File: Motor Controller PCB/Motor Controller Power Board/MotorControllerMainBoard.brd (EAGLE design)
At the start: 70 x 100 mm, 47 parts

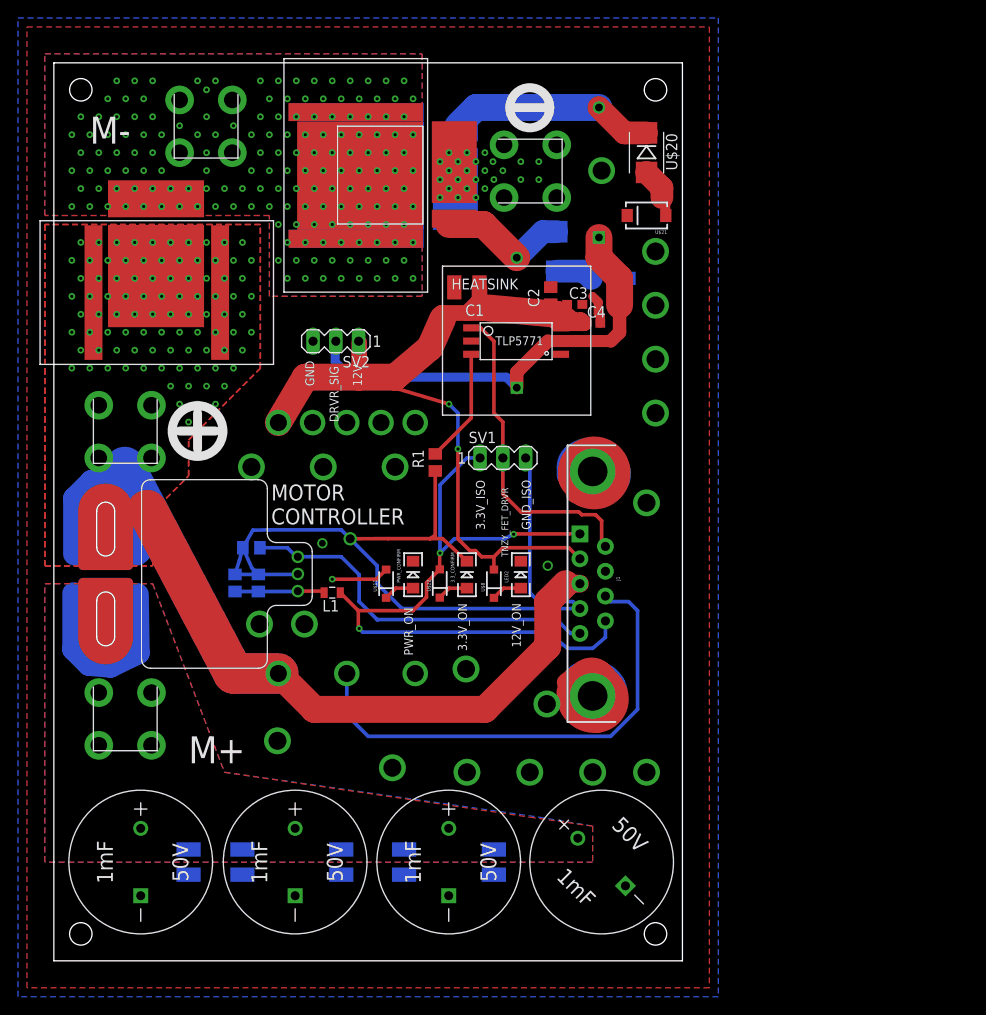
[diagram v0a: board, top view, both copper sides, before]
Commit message: Finishing Touches
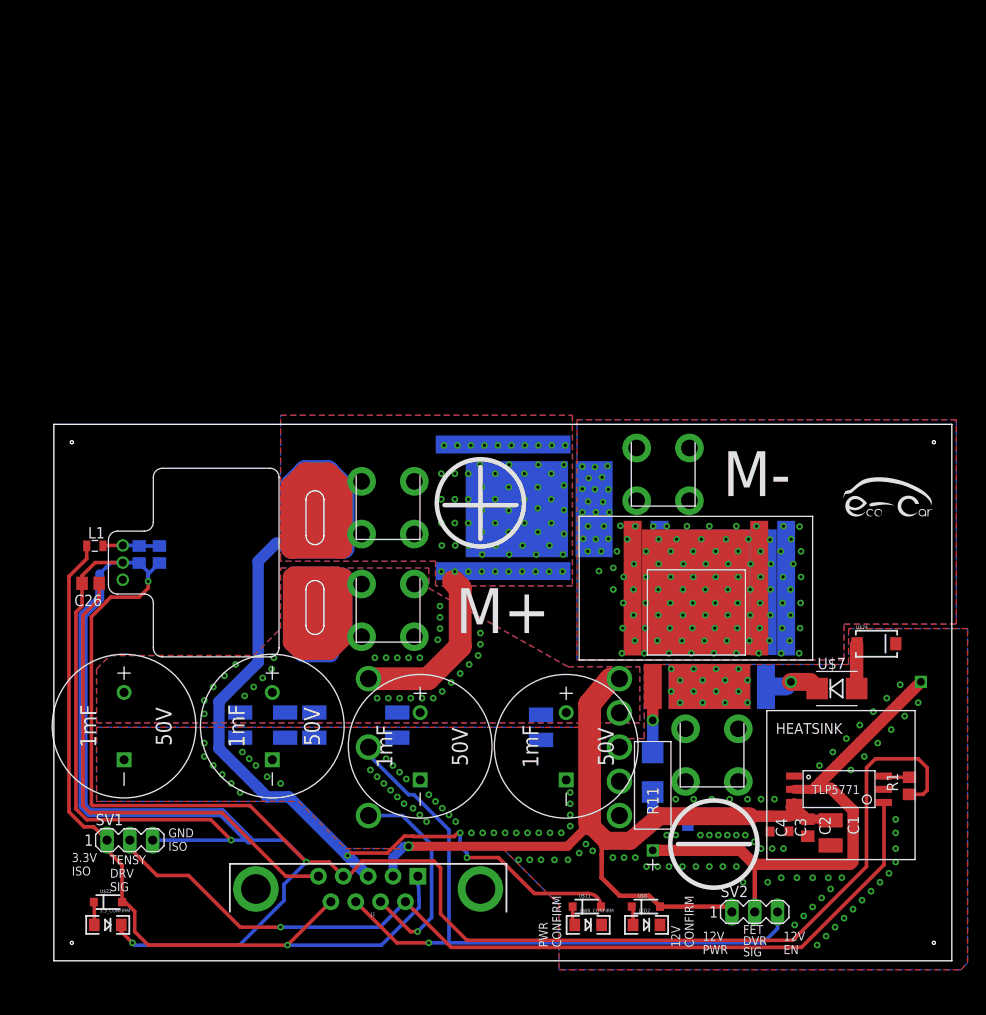
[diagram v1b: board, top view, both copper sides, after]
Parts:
- added U$26: (no value), Shell2015:LOGO
- moved SV2 78.8 mm to (78.0, 5.44), turned to 0 degrees
- moved C1 73.0 mm to (86.5, 14.2), turned to 270 degrees
- moved U$20 69.0 mm to (66.7, 21.0), flipped to the bottom
- moved R11 68.5 mm to (66.7, 26.8), flipped to the top
- moved U$21 67.9 mm to (68.5, 15.2), flipped to the bottom
- moved U$15 66.6 mm to (70.3, 20.0), turned to 0 degrees
- moved C2 65.8 mm to (84.0, 14.8), turned to 270 degrees
- moved U$12 64.0 mm to (64.9, 51.2)
- moved R1 63.9 mm to (95.3, 19.5)
- moved C3 62.6 mm to (81.9, 15.3), turned to 270 degrees
- moved U$2 61.7 mm to (74.5, 39.8), flipped to the bottom, turned to 0 degrees
- moved U$4 61.5 mm to (74.5, 41.5), flipped to the bottom, turned to 0 degrees
- moved U$25 61.3 mm to (79.4, 11.3)
- moved U$1 59.8 mm to (71.5, 39.8), flipped to the top, turned to 0 degrees
- moved U$3 59.5 mm to (71.5, 41.5), flipped to the top, turned to 0 degrees
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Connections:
- net ENABLE_12V: now also SV2.3
- net GND: no longer SV2.3
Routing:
- net GND_ISOLATED: track 100.4 -> 304.8 mm, vias 1 -> 4
- net TEENSY_FET_DRIVER_SIGNAL: track 35.8 -> 102.5 mm, vias 0 -> 1
- net INPUT_POWER(+): track 128.0 -> 165.4 mm, vias 92 -> 67
- net GND: track 56.9 -> 24.2 mm, vias 46 -> 135
- net ENABLE_12V: track 54.5 -> 77.2 mm, vias 0 -> 1
- net N$10: track 23.9 -> 7.36 mm
- net CURRENT_SENSOR_OUTPUT: track 41.4 -> 55.0 mm
- net 3.3V_ISOLATED: track 78.8 -> 92.1 mm, vias 3 -> 1
- net N$7: track 12.8 -> 2.90 mm
- net N$2: track 15.6 -> 6.22 mm
- net FET_DRIVER_SIGNAL: track 50.3 -> 58.5 mm
- net N$6: track 10.0 -> 6.34 mm
- net N$4: track 5.69 -> 3.76 mm
- net N$9: track 3.45 -> 2.10 mm
- net N$17: track 3.45 -> 2.13 mm
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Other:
- board size 70 x 100 mm -> 100 x 59.8 mm
- board text added: "12V CONFIRM"
- board text added: "12V EN"
- board text added: "12V PWR"
- board text added: "3.3V ISO"
- board text added: "DC Motor Controller MAX 30V, 40A"
- board text added: "FET DVR SIG"
- board text added: "GND ISO"
- board text added: "PWR CONFIRM"
- board text added: "TENSY DRV SIG"
- board text removed: "12V"
- board text removed: "12V_ON"
- board text removed: "2018 Koltin Kosik-Harvey"
- board text removed: "3.3V_ISO"
- board text removed: "3.3V_ON"
- board text removed: "DRVR_SIG"
- board text removed: "GND"
- board text removed: "GND_ISO"
- board text removed: "MOTOR CONTROLLER"
- board text removed: "PWR_ON"
- board text removed: "TNZY_FET_DRVR"
